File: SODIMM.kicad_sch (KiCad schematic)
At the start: 5 parts, among them CN1 YXT-BB10-50P-02, CN2 YXT-BB10-50P-02, CN3 YXT-BB10-50P-02, U6 Compute_Module_4_Connectors, U7 Compute_Module_4_Functional

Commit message: changed some ethernet stuff
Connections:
- net GND: now also CN2.12, CN2.16, CN2.3, CN2.6, CN2.9, CN3.10, CN3.14, CN3.17, CN3.45, CN3.5
- net ENET_MDI0+: now reaches CN2.1
- net ENET_MDI3+: now reaches CN2.10
- net ENET_MDI3-: now reaches CN2.11
- net ENET_LED1: now reaches CN2.13
- net ENET_LED0: now reaches CN2.14
- net ENET_LED2: now reaches CN2.15
- net ENET_MDI0-: now reaches CN2.2
- net ENET_MDI1+: now reaches CN2.4
- net ENET_MDI1-: now reaches CN2.5
- net ENET_MDI2+: now reaches CN2.7
- net ENET_MDI2-: now reaches CN2.8
- net JTAG_MS: now reaches CN3.1
- net PA8: now reaches CN3.11
- net PA9: now reaches CN3.12
- net PA10: now reaches CN3.13
- net TWI0_SCK: now reaches CN3.15
- net TWI0_SDA: now reaches CN3.16
- net UART3_TX: now reaches CN3.18
- net UART3_RX: now reaches CN3.19
- net JTAG_CK: now reaches CN3.2
- net UART3_RTS: now reaches CN3.20
- net UART3_CTS: now reaches CN3.21
- net JTAG_DO: now reaches CN3.3
- net JTAG_DI: now reaches CN3.4
- net SPI0_CS: now reaches CN3.41
- net SPI0_CLK: now reaches CN3.42
- net SPI0_MISO: now reaches CN3.43
- net SPI0_MOSI: now reaches CN3.44
- net PA21: now reaches CN3.46
- net PA20: now reaches CN3.47
- net PA19: now reaches CN3.48
- net PA18: now reaches CN3.49
- net PA17: now reaches CN3.50
- net PA4: now reaches CN3.6
- net PA5: now reaches CN3.7
- net PA6: now reaches CN3.8
- net PA7: now reaches CN3.9
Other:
- note added: "Connections for - Power \, USB (0-3) \, HDMI \. Ethernet \, SD \, Audio \, IO \, JTAG"
- note removed: "Connections for - Power \, USB (0-3) \, HDMI - Ethernet \, SD - Audio"
- moved on the sheet: CN2, CN3, U7B, U7D, U7E, U7F, U7G, U7I, U7J

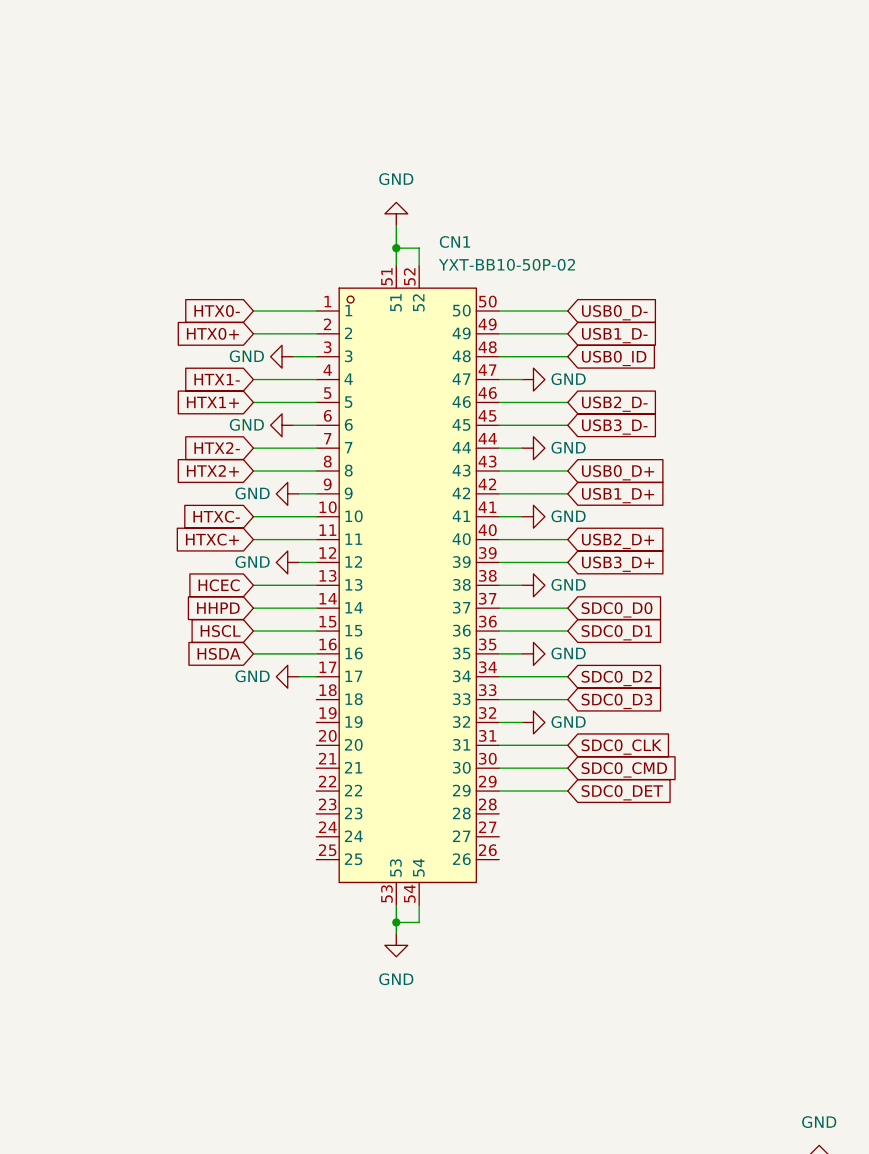
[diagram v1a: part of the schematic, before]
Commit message: power changes
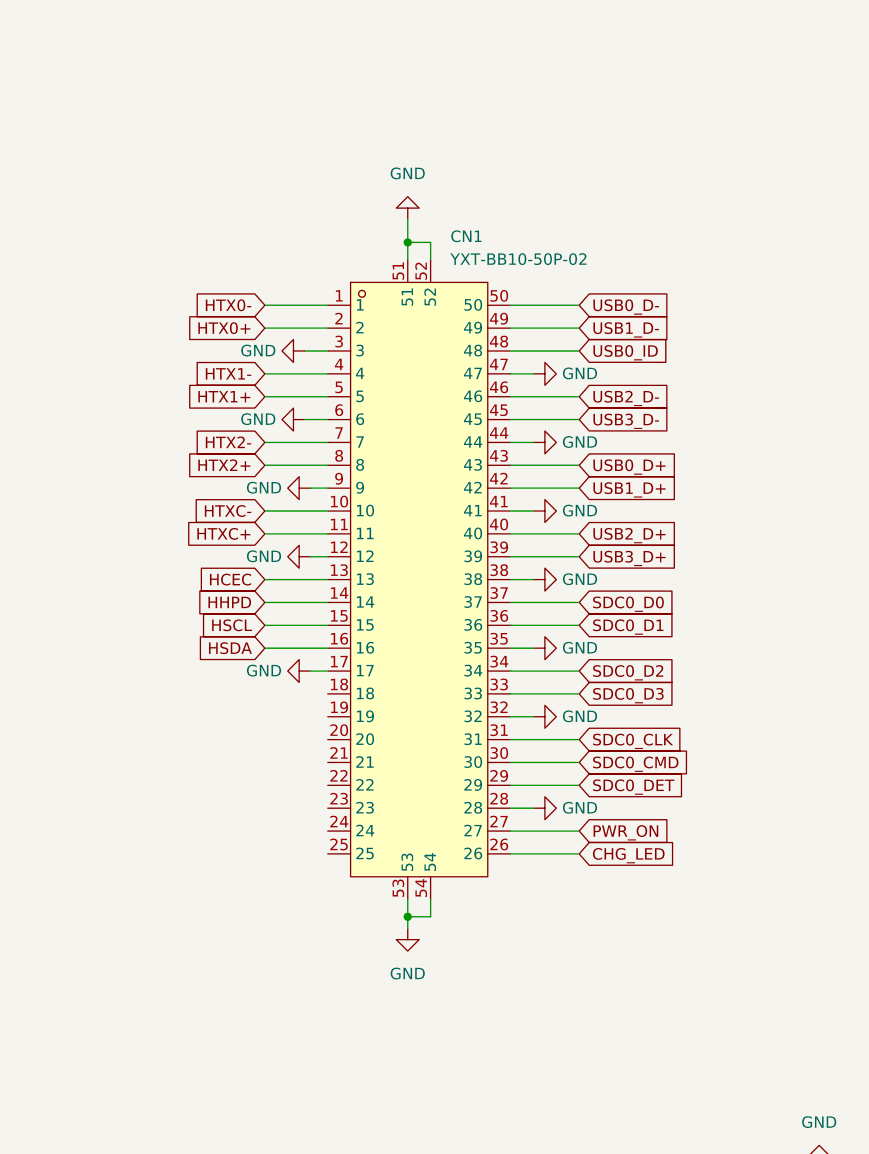
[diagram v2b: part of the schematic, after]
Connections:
- net GND: now also CN1.28
- net CHG_LED: now reaches CN1.26
- net PWR_ON: now reaches CN1.27
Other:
- moved on the sheet: CN1
